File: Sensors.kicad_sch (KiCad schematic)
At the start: 8 parts, among them U18 LTR-303ALS-01, U7 BME280

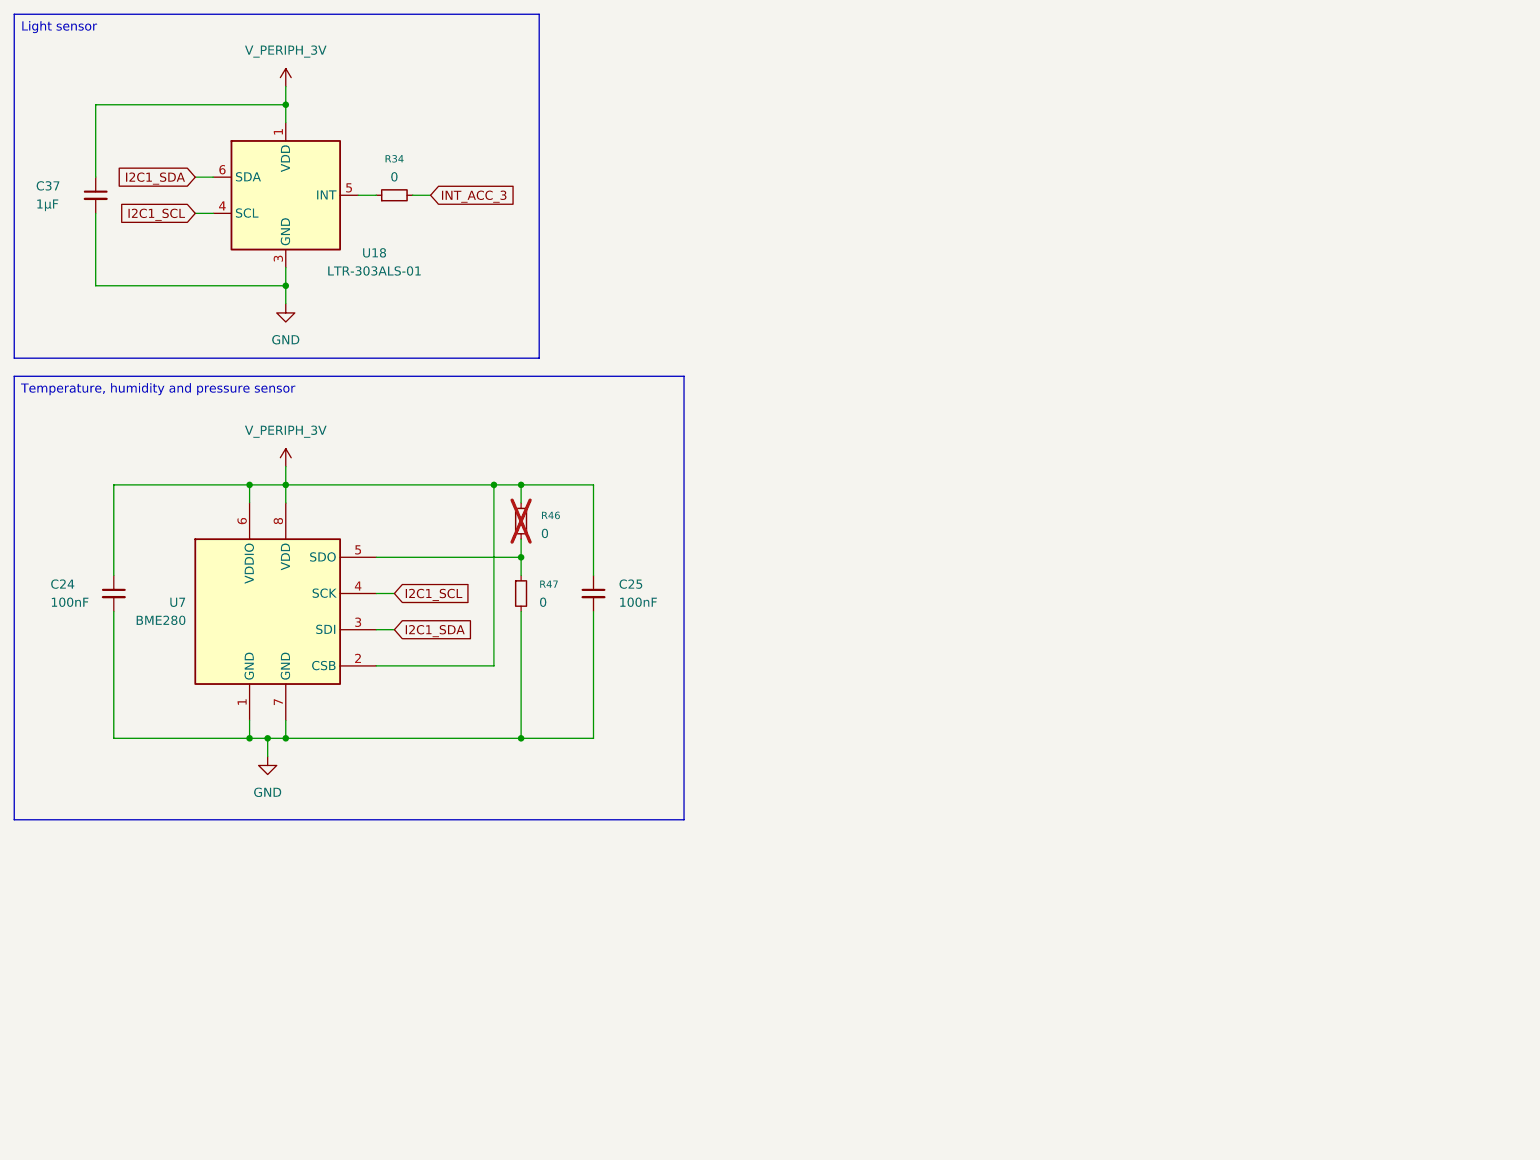
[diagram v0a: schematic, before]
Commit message: Continue filling schematics
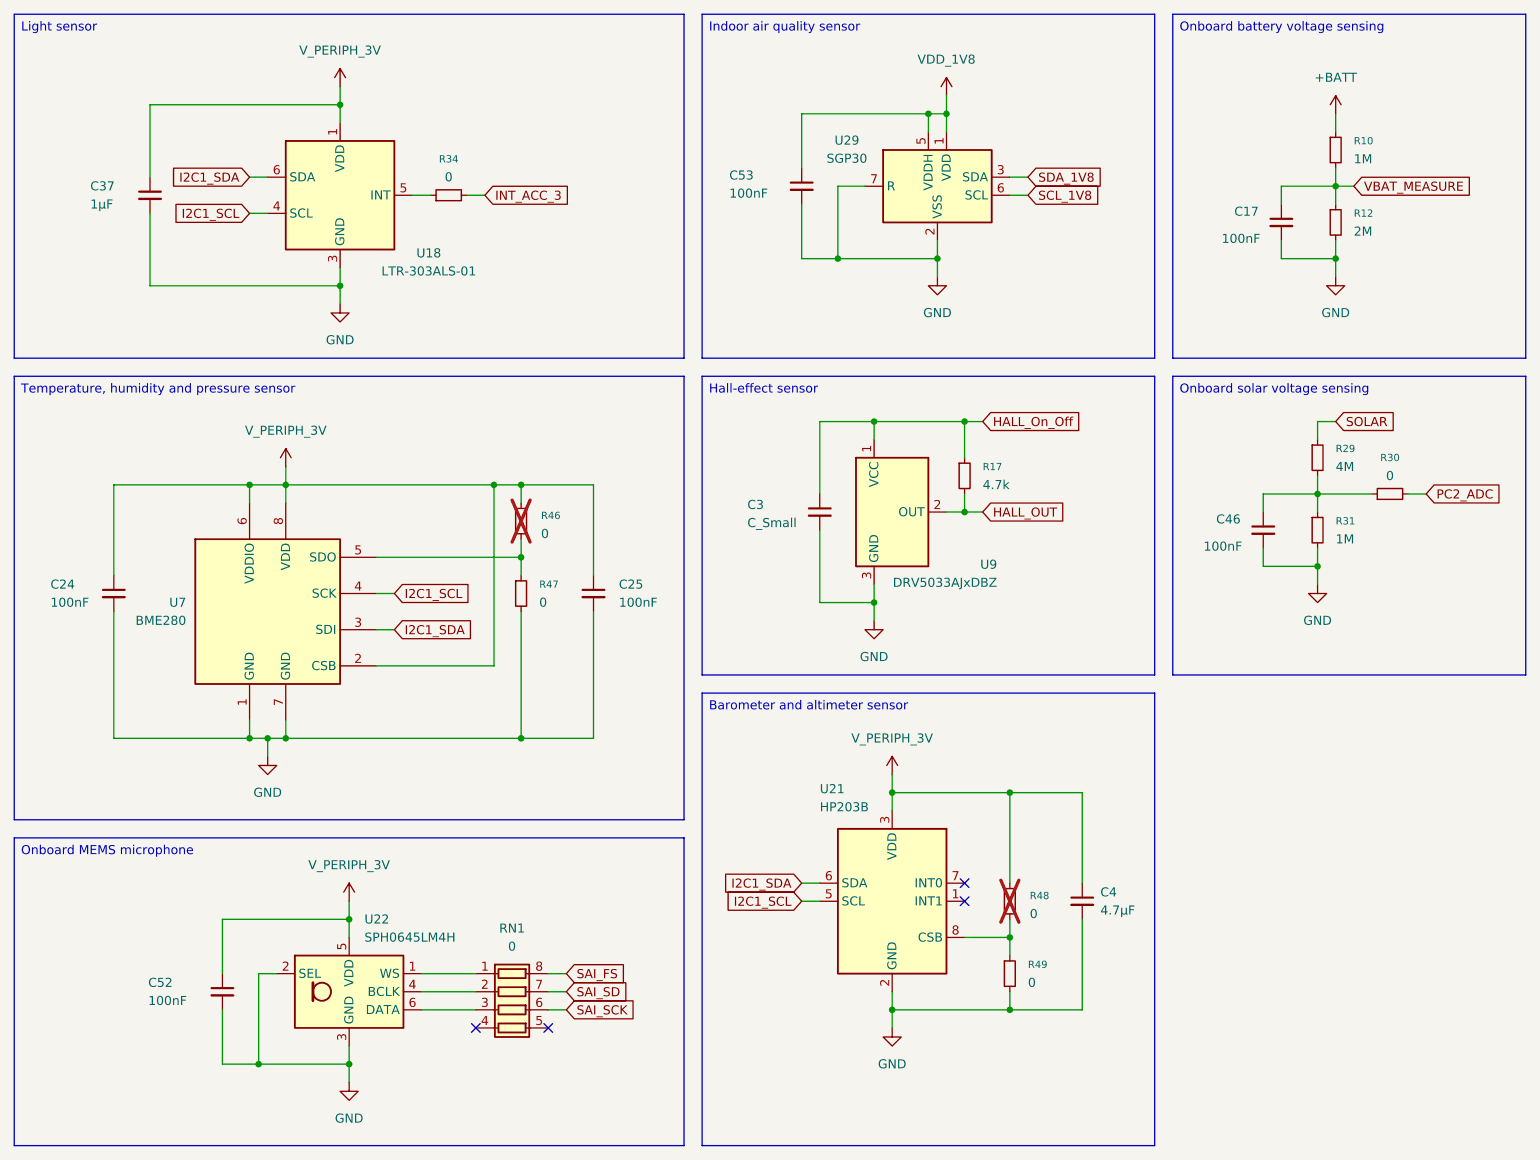
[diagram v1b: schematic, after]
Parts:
- added C17, C46, C52, C53: 100nF, symbol Device:C_Small
- added C3: C_Small, symbol Device:C_Small
- added C4: 4.7µF, symbol Device:C_Small
- added R10, R31: 1M, symbol Device:R_Small
- added R12: 2M, symbol Device:R_Small
- added R17: 4.7k, symbol Device:R_Small
- added R29: 4M, symbol Device:R_Small
- added R30, R48, R49: 0, symbol Device:R_Small
- added RN1: 0, symbol Device:R_Pack04
- added U21: HP203B, Package_LGA:NXP_LGA-8_3x5mm_P1.25mm_H1.1mm, symbol HOPERF_HP203B:HP203B
- added U22: SPH0645LM4H, Sensor_Audio:Knowles_SPH0645LM4H-6_3.5x2.65mm, symbol Sensor_Audio:SPH0645LM4H
- added U29: SGP30, footprints:Sensirion_DFN-6-1EP_2.44x2.44mm_P0.8mm, symbol Sensirion_SGP30:SGP30
- added U9: DRV5033AJxDBZ, Package_TO_SOT_SMD:SOT-23, symbol Sensor_Magnetic:DRV5033AJxDBZ
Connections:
- net GND: now also C17.2, C3.2, C4.2, C46.2, C52.2, C53.2, R12.2, R31.2, R49.2, U21.2 (GND), U22.2 (SEL), U22.3 (GND), U29.2 (VSS), U29.7 (R), U29.9 (VSS), U9.3 (GND)
- net I2C1_SCL: now also U21.5 (SCL)
- net I2C1_SDA: now also U21.6 (SDA)
- net V_PERIPH_3V: now also C4.1, C52.1, R48.1, U21.3 (VDD), U22.5 (VDD)
- new net: RN1.1 (R1.1), U22.1 (WS)
- new net: RN1.2 (R2.1), U22.4 (BCLK)
- new net: RN1.3 (R3.1), U22.6 (DATA)
- new net: R48.2, R49.1, U21.8 (CSB)
- new net: C46.1, R29.2, R30.1, R31.1
- new net +BATT: R10.1
- new net HALL_OUT: R17.2, U9.2 (OUT)
- new net HALL_On_Off: C3.1, R17.1, U9.1 (VCC)
- new net PC2_ADC: R30.2
- new net SAI_FS: RN1.8 (R1.2)
- new net SAI_SCK: RN1.6 (R3.2)
- new net SAI_SD: RN1.7 (R2.2)
- new net SCL_1V8: U29.6 (SCL)
- new net SDA_1V8: U29.3 (SDA)
- new net SOLAR: R29.1
- new net VBAT_MEASURE: C17.1, R10.2, R12.1
- new net VDD_1V8: C53.1, U29.1 (VDD), U29.5 (VDDH)
- no-connect marks 0 -> 4
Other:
- company: (none) -> //piernov
- moved on the sheet: C37, R34, U18
